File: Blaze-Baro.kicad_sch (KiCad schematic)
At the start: 5 parts, among them U1 QTStemma_M, U2 MS5611

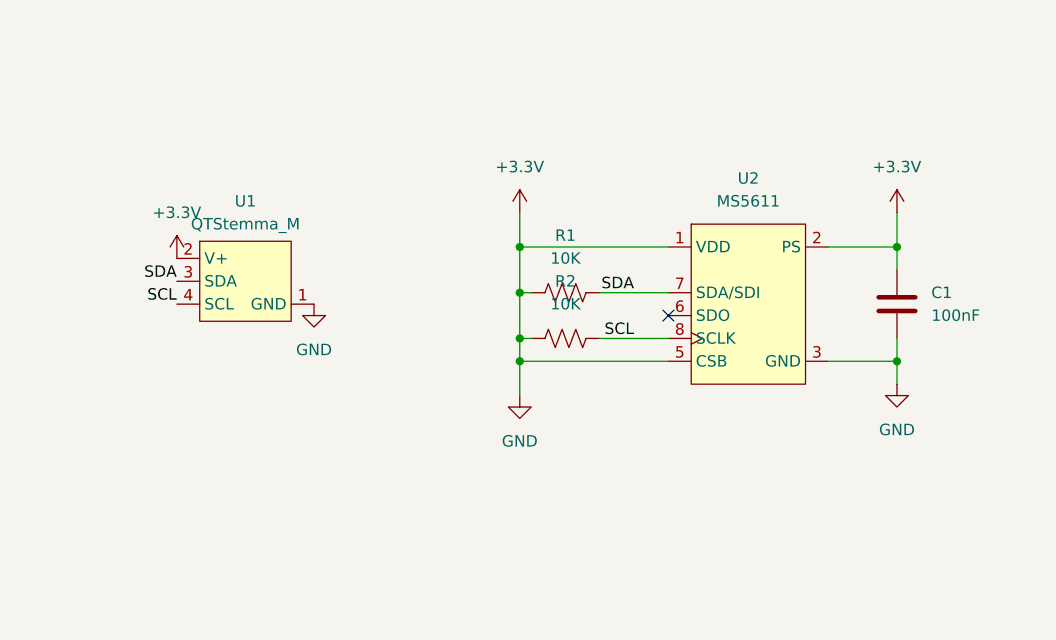
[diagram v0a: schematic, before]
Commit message: push recent changes added stemma qt footprint
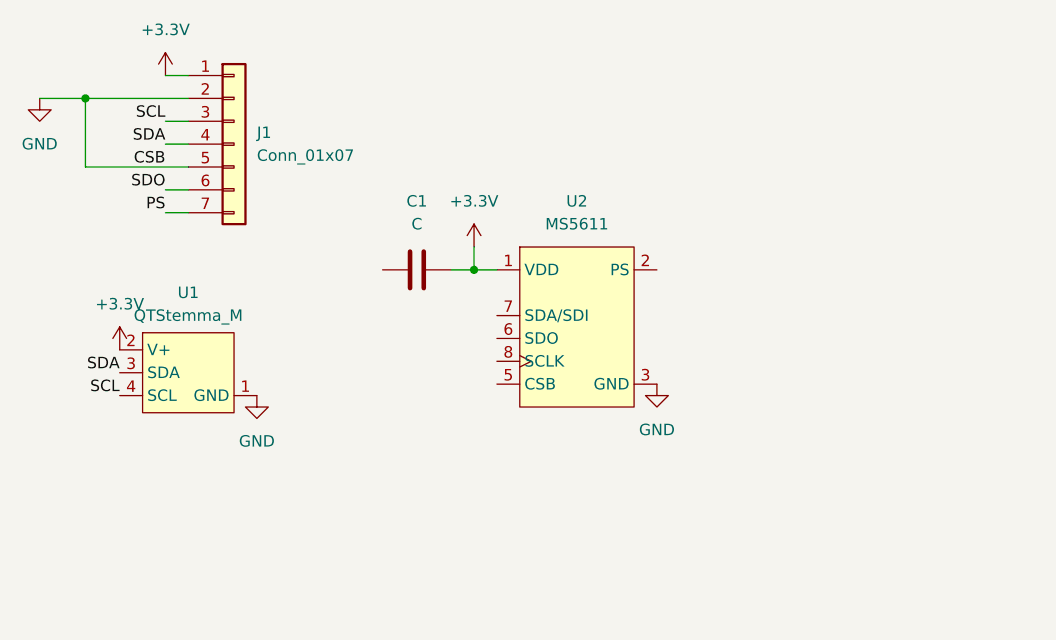
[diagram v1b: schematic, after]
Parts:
- removed R1, R2: 10K, Resistor_SMD:R_0201_0603Metric, symbol Device:R_US
- added J1: Conn_01x07, symbol Connector_Generic:Conn_01x07
- C1: value 100nF -> C; footprint Capacitor_SMD:C_0805_2012Metric -> (none)
- U1: footprint (none) -> Connector_JST:JST_SH_SM02B-SRSS-TB_1x02-1MP_P1.00mm_Horizontal
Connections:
- net +3.3V: now also J1.1 (Pin_1); no longer C1.1, U1.1 (GND), U2.2 (PS), U2.3 (GND), U2.4 (CSB), U2.5 (CSB)
- net SCL: now also J1.3 (Pin_3); no longer U2.8 (SCLK)
- net SDA: now also J1.4 (Pin_4); no longer U2.7 (SDA/SDI)
- new net: U2.4 (CSB), U2.5 (CSB)
- new net GND: J1.2 (Pin_2), J1.5 (Pin_5), U1.1 (GND), U2.3 (GND)
- new net PS: J1.7 (Pin_7)
- new net SDO: J1.6 (Pin_6)
- no-connect marks 1 -> 0
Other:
- moved on the sheet: U1, U2

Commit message: Redid schematic
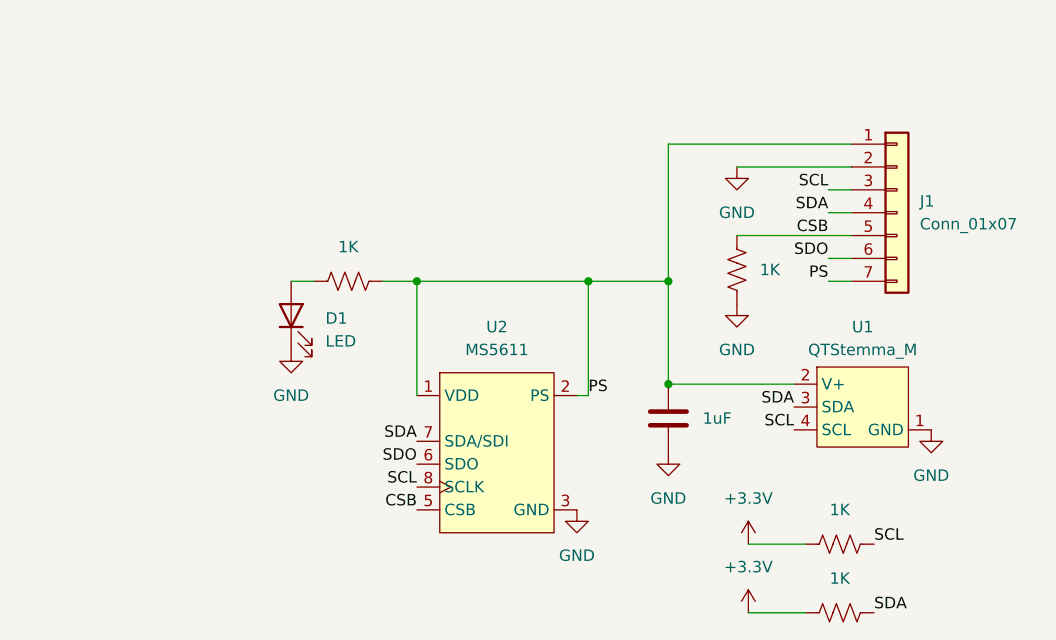
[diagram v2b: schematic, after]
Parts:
- added D1: LED, symbol Device:LED
- added R1, R2, R3, R4: 1K, symbol Device:R_US
- C1: value C -> 1uF
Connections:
- net +3.3V: now also R3.2, R4.2; no longer C1.2, J1.1 (Pin_1), U1.2 (V+), U2.1 (VDD)
- net GND: now also C1.1, D1.1 (K), R2.2; no longer J1.5 (Pin_5)
- net PS: now also C1.2, J1.1 (Pin_1), U1.2 (V+), U2.1 (VDD), U2.2 (PS), R1.1
- net SCL: now also U2.8 (SCLK), R3.1
- net SDA: now also U2.7 (SDA/SDI), R4.1
- net SDO: now also U2.6 (SDO)
- net CSB: now reaches U2.4 (CSB), U2.5 (CSB)
- net CSB: now also J1.5 (Pin_5), R2.1
- new net: D1.2 (A), R1.2
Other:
- moved on the sheet: J1, U1, U2
